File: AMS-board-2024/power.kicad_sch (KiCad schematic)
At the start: 67 parts, among them Q109 DMT6007LFGQ, Q110 BSS308PE, Q111 2N7002K-AU, Q112 2N7002K-AU, Q113 DMT6007LFGQ, Q114 2N7002K-AU, U18 UCC12040, U19 AP74700QW6-7, U20 VOMA617A, U21 LM5060, U22 LMR33630APCQRNXRQ1

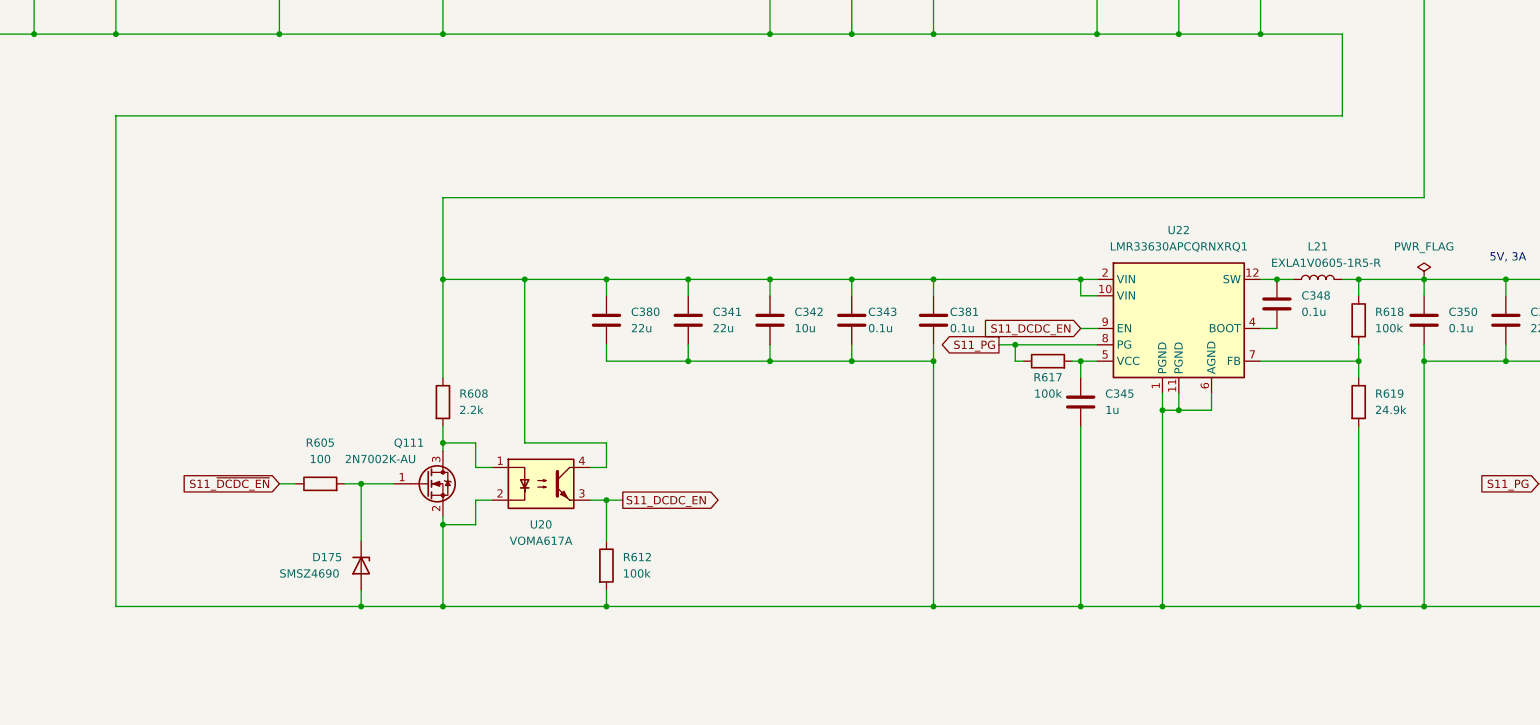
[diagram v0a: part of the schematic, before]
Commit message: DCDC ENABLE周辺回路修正
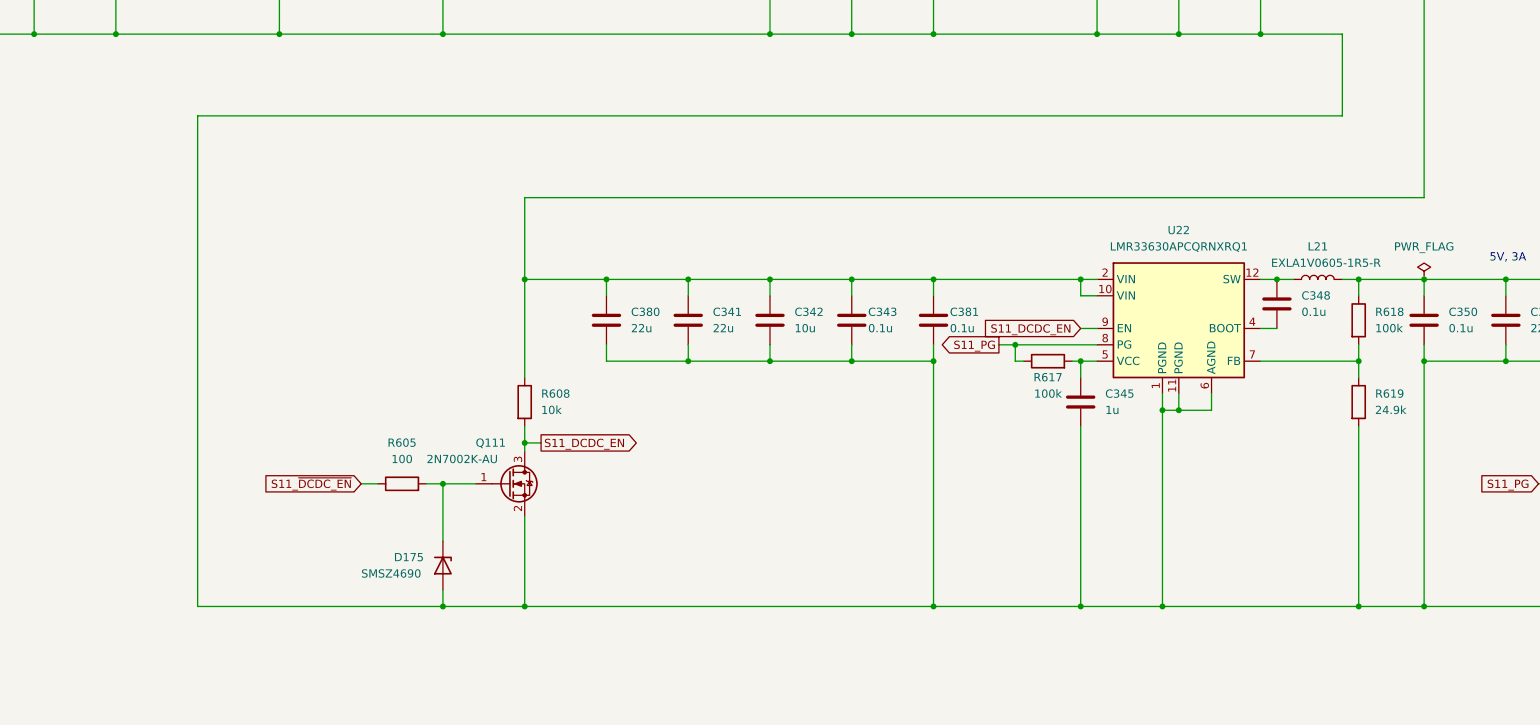
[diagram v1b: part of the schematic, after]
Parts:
- removed R612: 100k, Resistor_SMD:R_0402_1005Metric, symbol Device:R
- removed U20: VOMA617A, ProjectEV:Package_SOP-4_4.57x4.92mm_P2.54mm_VOMA617A, symbol ProjectEV:Isolator_VOMA617A
- R608: value 2.2k -> 10k
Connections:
- net S11_DCDC_EN: now also Q111.3 (D), R608.2
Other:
- moved on the sheet: D175, Q111, R605, R608
